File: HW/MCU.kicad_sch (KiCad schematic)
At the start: 7 parts, among them U6 STM32C031KxTx, U7 STM32C031KxUx

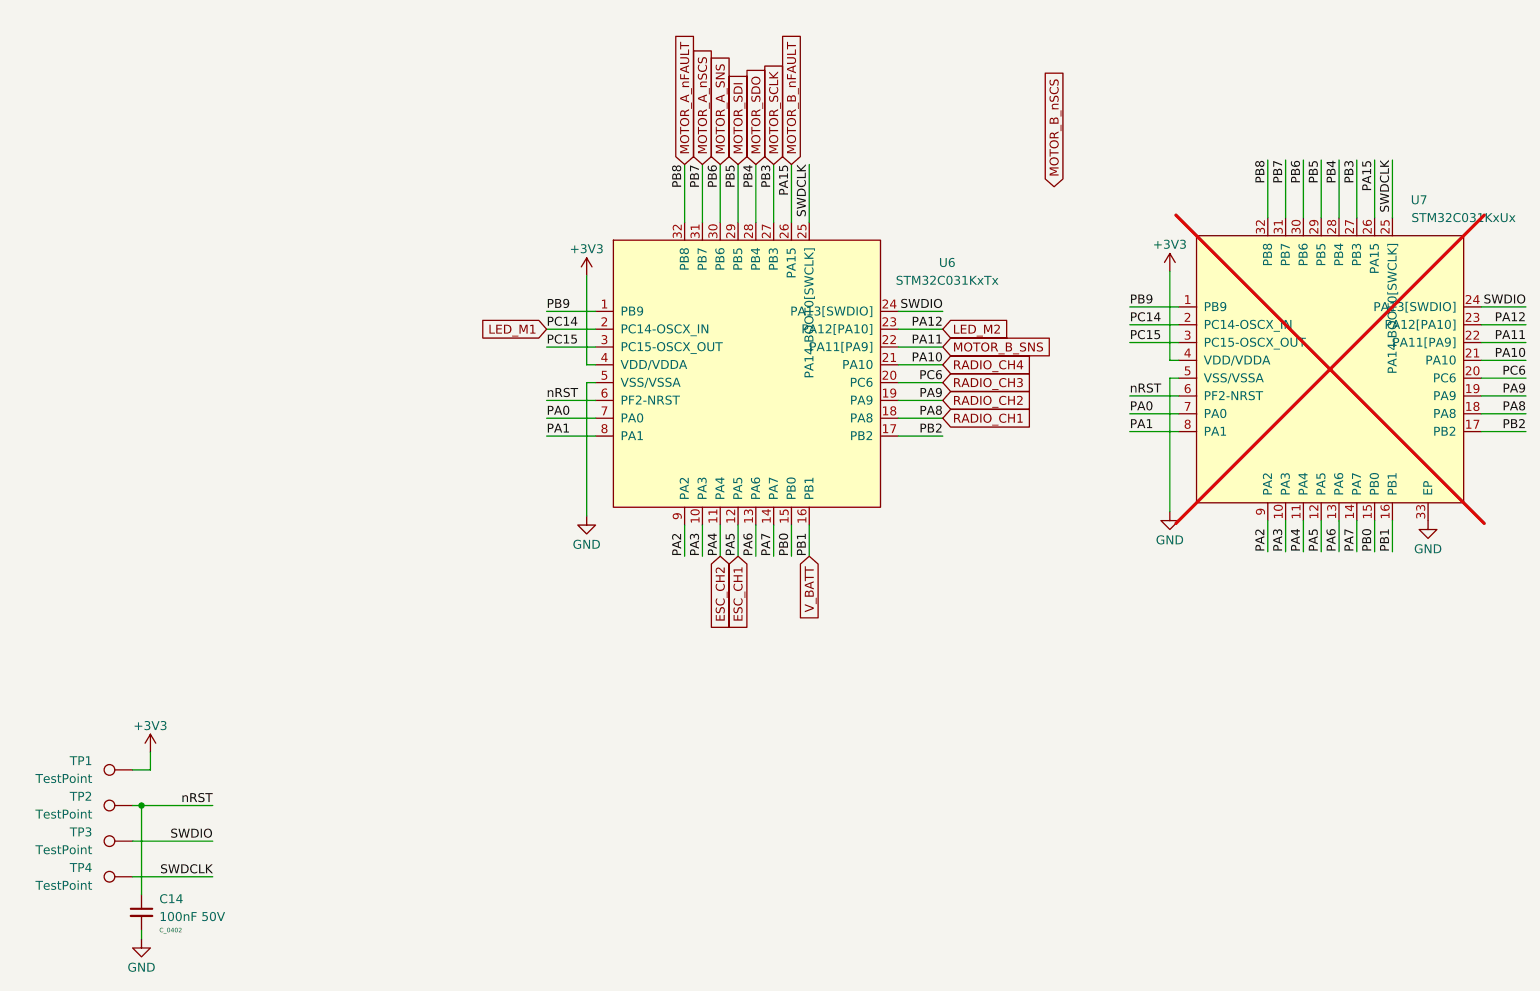
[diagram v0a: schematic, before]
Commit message: Finish Tracking and Release For MFG
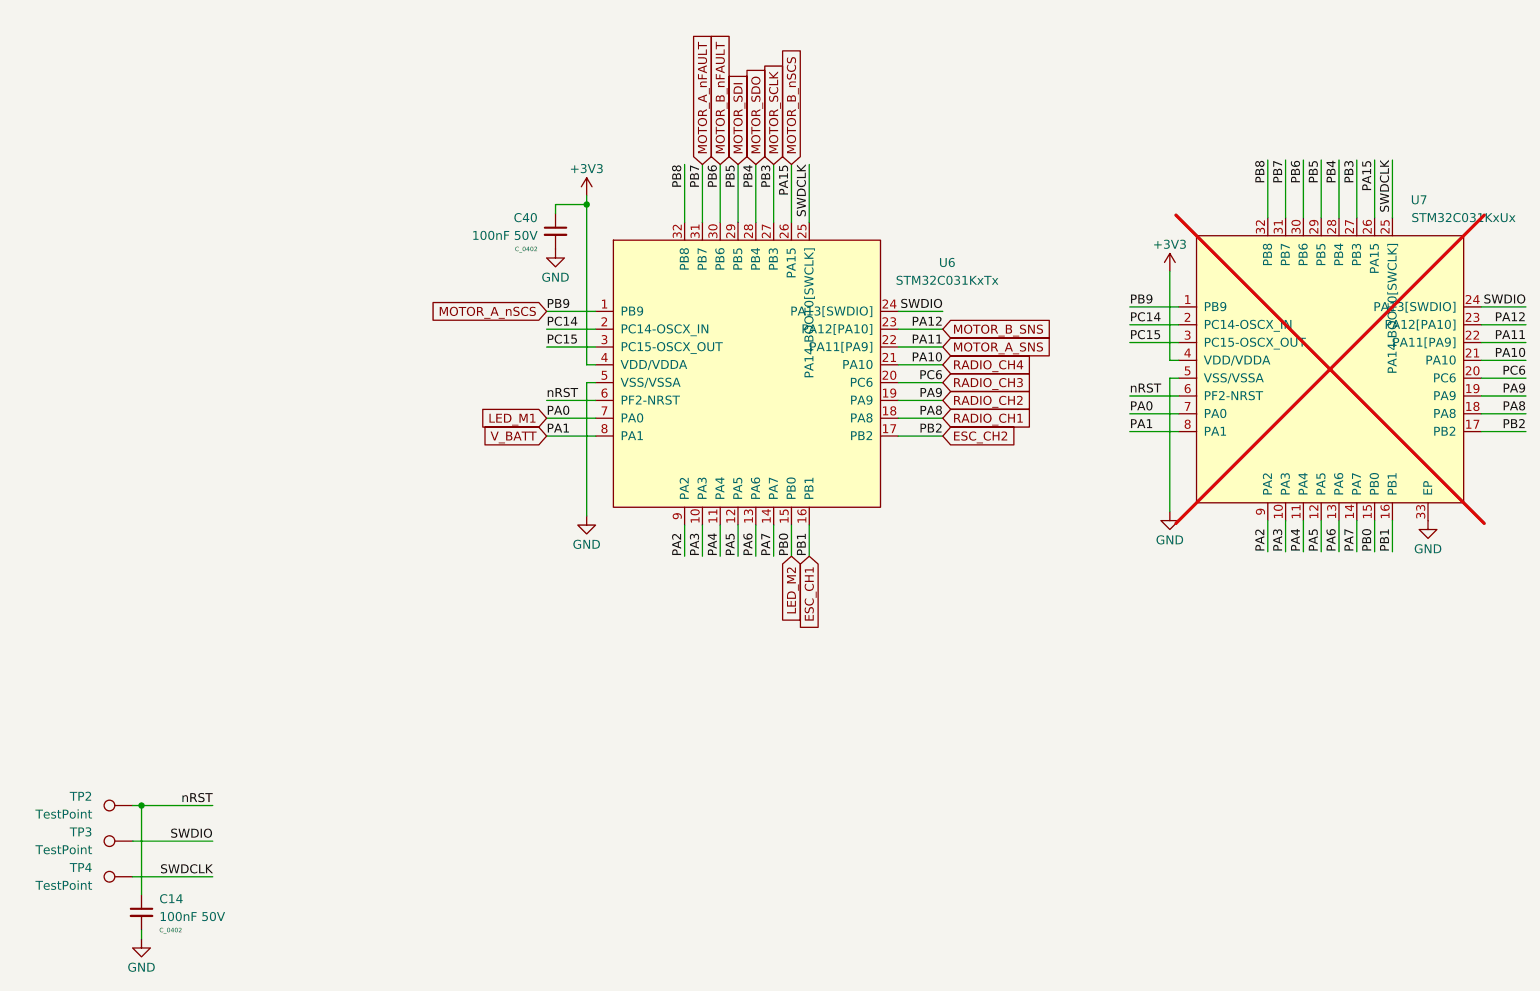
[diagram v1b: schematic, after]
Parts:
- removed TP1: TestPoint, TestPoint:TestPoint_Pad_D1.5mm, symbol Connector:TestPoint
- added C40: 100nF 50V, C_Capacitor:C_0402, symbol C_Capacitor:C_0402
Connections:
- net PA0 is gone; now on net LED_M1: U6.7 (PA0), U7.7 (PA0)
- net PA1 is gone; now on net V_BATT: U6.8 (PA1), U7.8 (PA1)
- net PB0 is gone; now on net LED_M2: U6.15 (PB0), U7.15 (PB0)
- net PB2 is gone; now on net ESC_CH2: U6.17 (PB2), U7.17 (PB2)
- net PB9 is gone; now on net MOTOR_A_nSCS: U6.1 (PB9), U7.1 (PB9)
- net +3V3: now also C40.1
- net ESC_CH1: now also U6.16 (PB1), U7.16 (PB1); no longer U6.12 (PA5), U7.12 (PA5)
- net ESC_CH2: no longer U6.11 (PA4), U7.11 (PA4)
- net GND: now also C40.2
- net LED_M1: no longer U6.2 (PC14-OSCX_IN), U7.2 (PC14-OSCX_IN)
- net LED_M2: no longer U6.23 (PA12[PA10]), U7.23 (PA12[PA10])
- net MOTOR_A_SNS: now also U6.22 (PA11[PA9]), U7.22 (PA11[PA9]); no longer U6.30 (PB6), U7.30 (PB6)
- net MOTOR_A_nFAULT: now also U6.31 (PB7), U7.31 (PB7); no longer U6.32 (PB8), U7.32 (PB8)
- net MOTOR_A_nSCS: no longer U6.31 (PB7), U7.31 (PB7)
- net MOTOR_B_SNS: now also U6.23 (PA12[PA10]), U7.23 (PA12[PA10]); no longer U6.22 (PA11[PA9]), U7.22 (PA11[PA9])
- net MOTOR_B_nFAULT: now also U6.30 (PB6), U7.30 (PB6); no longer U6.26 (PA15), U7.26 (PA15)
- net MOTOR_B_nSCS: now also U6.26 (PA15), U7.26 (PA15)
- net V_BATT: no longer U6.16 (PB1), U7.16 (PB1)
- new net PA4: U6.11 (PA4), U7.11 (PA4)
- new net PA5: U6.12 (PA5), U7.12 (PA5)
- new net PB8: U6.32 (PB8), U7.32 (PB8)
- new net PC14: U6.2 (PC14-OSCX_IN), U7.2 (PC14-OSCX_IN)
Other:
- title: KAKAPO ESC - 20A -> KAKAPO - 20A
